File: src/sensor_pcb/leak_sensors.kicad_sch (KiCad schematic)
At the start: 36 parts, among them Q1 NPN BJT 40V 200mA, Q2 NPN BJT 40V 200mA, Q3 NPN BJT 40V 200mA, Q4 NPN BJT 40V 200mA, Q5 NPN BJT 40V 200mA, Q6 NPN BJT 40V 200mA

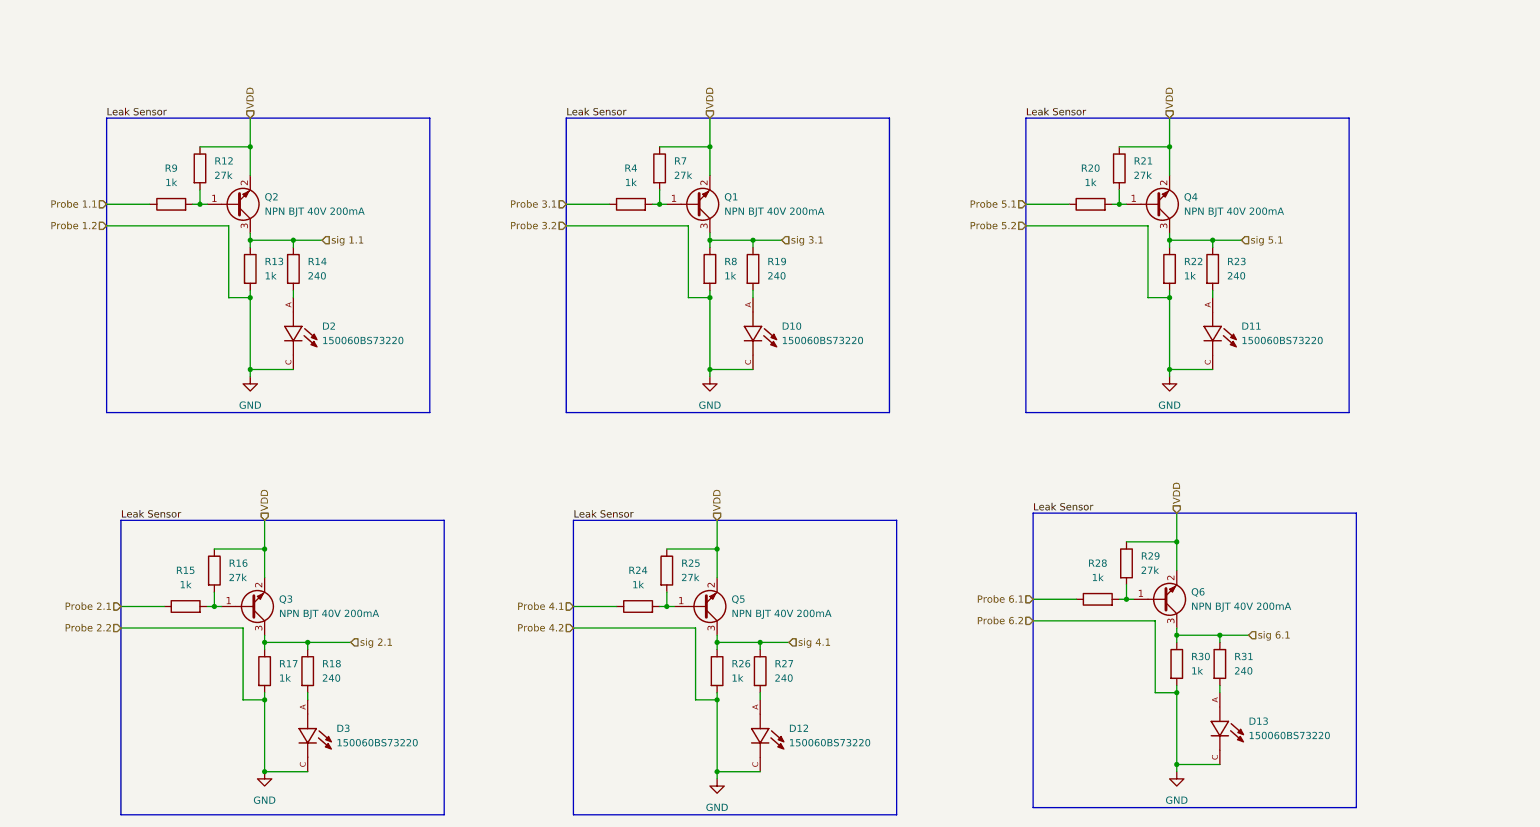
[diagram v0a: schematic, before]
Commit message: tuesday changes
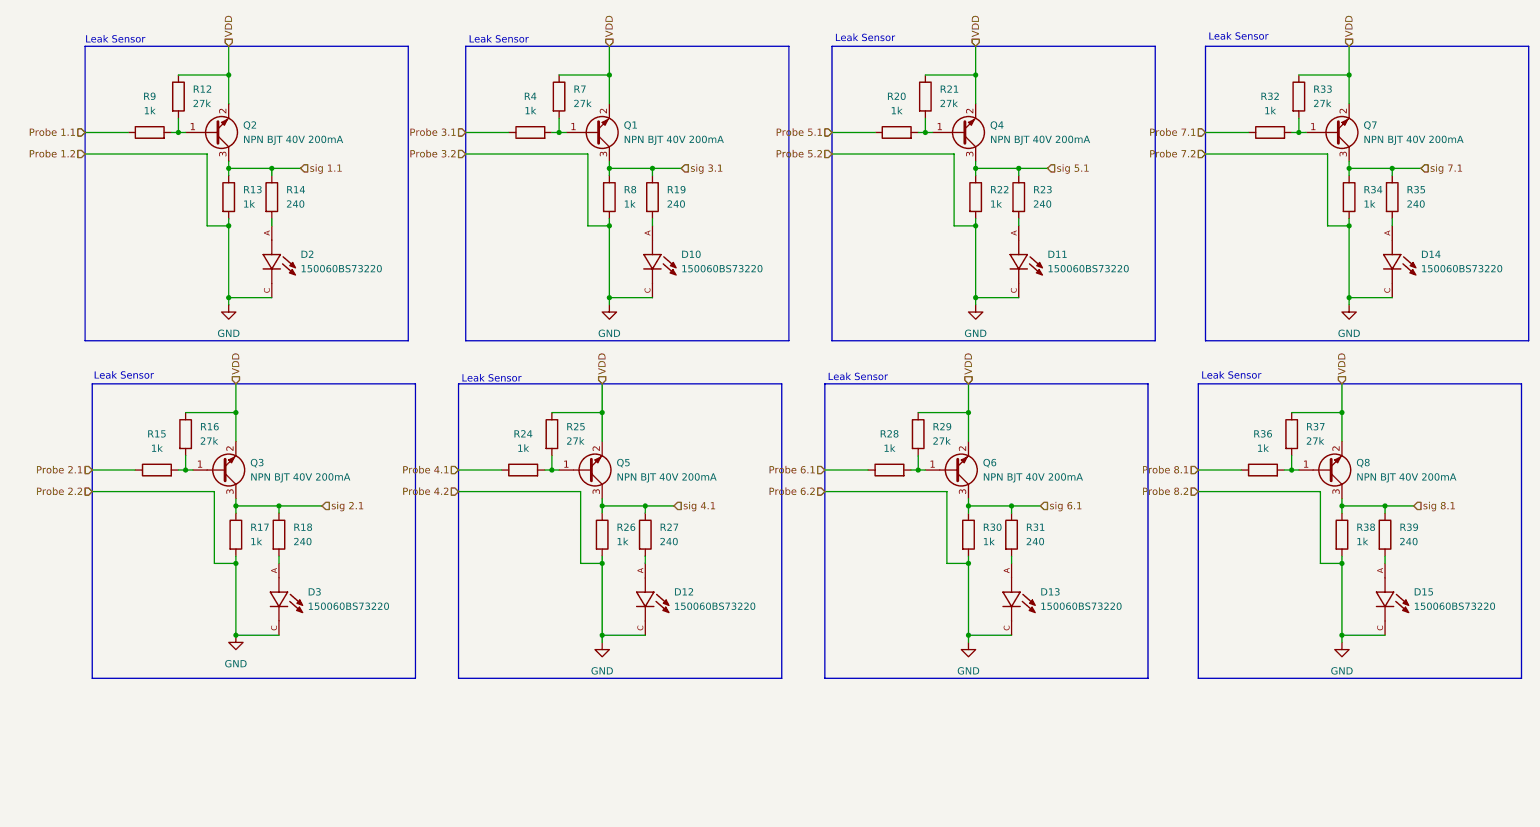
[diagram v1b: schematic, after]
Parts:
- added D14, D15: 150060BS73220, dz_dio:LED_0603, symbol #dzdb:s_dio/D-WUR-150060BS73220
- added Q7, Q8: NPN BJT 40V 200mA, Package_TO_SOT_SMD:SOT-23, symbol #dzdb:s_misc/Q-NPN-200-SOT23
- added R32, R34, R36, R38: 1k, Resistor_SMD:R_0603_1608Metric, symbol #dzdb:g_res/R-1k-0603
- added R33, R37: 27k, Resistor_SMD:R_0603_1608Metric, symbol #dzdb:g_res/R-27k-0603
- added R35, R39: 240, Resistor_SMD:R_0603_1608Metric, symbol #dzdb:g_res/R-240-0603
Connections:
- net GND: now also D14.C, D15.C, R34.2, R38.2
- net VDD: now also Q7.2 (E), Q8.2 (E), R33.1, R37.1
- new net: Q7.1 (B), R32.2, R33.2
- new net: D15.A, R39.2
- new net: D14.A, R35.2
- new net: Q8.1 (B), R36.2, R37.2
- new net Probe 7.1: R32.1
- new net Probe 8.1: R36.1
- new net sig 7.1: Q7.3 (C), R34.1, R35.1
- new net sig 8.1: Q8.3 (C), R38.1, R39.1
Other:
- note added: "Leak Sensor"
- moved on the sheet: D10, D11, D12, D13, D2, D3, Q1, Q2, Q3, Q4, Q5, Q6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
